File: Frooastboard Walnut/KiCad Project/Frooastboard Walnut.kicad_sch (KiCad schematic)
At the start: 159 parts, among them SW1 SW_Push, U1 ATmega32U4-A, Y1 Crystal_GND24_Small

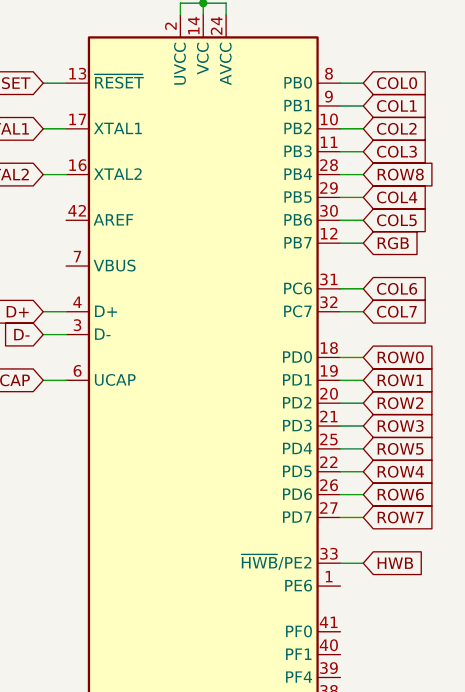
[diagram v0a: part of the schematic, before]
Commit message: backup
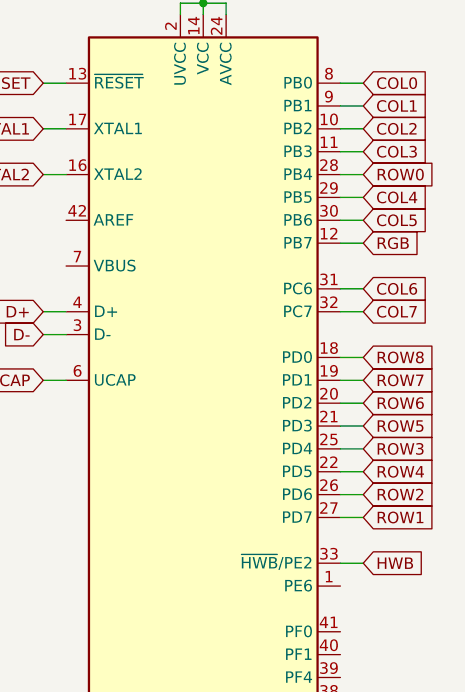
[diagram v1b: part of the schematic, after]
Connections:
- net ROW0: now also U1.28 (PB4); no longer U1.18 (PD0)
- net ROW1: now also U1.27 (PD7); no longer U1.19 (PD1)
- net ROW2: now also U1.26 (PD6); no longer U1.20 (PD2)
- net ROW3: now also U1.25 (PD4); no longer U1.21 (PD3)
- net ROW5: now also U1.21 (PD3); no longer U1.25 (PD4)
- net ROW6: now also U1.20 (PD2); no longer U1.26 (PD6)
- net ROW7: now also U1.19 (PD1); no longer U1.27 (PD7)
- net ROW8: now also U1.18 (PD0); no longer U1.28 (PB4)

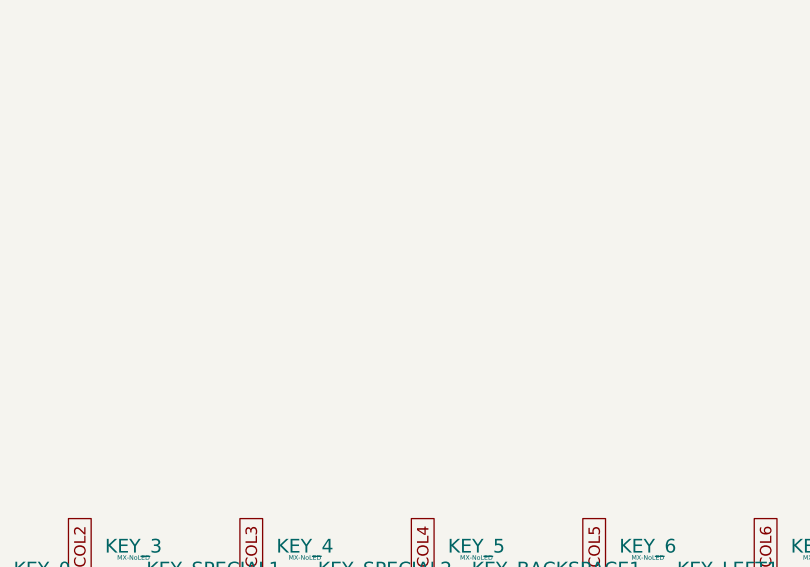
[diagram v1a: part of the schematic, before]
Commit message: Finished Basic Layout
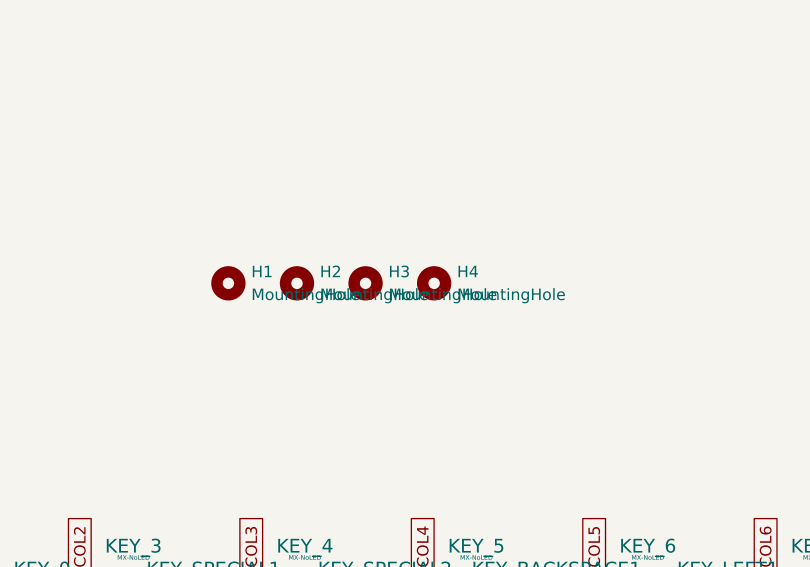
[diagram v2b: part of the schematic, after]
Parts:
- added H1, H2, H3, H4: MountingHole, MountingHole:MountingHole_3.2mm_M3_DIN965, symbol Mechanical:MountingHole
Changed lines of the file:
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@@
     (pin "2")
+  )
+  (symbol (lib_id "Mechanical:MountingHole") (at 116.84 74.93 0) (unit 1)
+    (in_bom yes) (on_board yes) (fields_autoplaced)
+    (property "Reference" "H4" (id 0) (at 119.38 73.6599 0)
+      (effects (font (size 1.27 1.27)) (justify left))
+    )
+    (property "Value" "MountingHole" (id 1) (at 119.38 76.1999 0)
+      (effects (font (size 1.27 1.27)) (justify left))
+    )
+    (property "Footprint" "MountingHole:MountingHole_3.2mm_M3_DIN965" (id 2) (at 116.84 74.93 0)
+      (effects (font (size 1.27 1.27)) hide)
+    )
+    (property "Datasheet" "~" (id 3) (at 116.84 74.93 0)
+      (effects (font (size 1.27 1.27)) hide)
+    )
   )
   (symbol (lib_id "MX_Alps_Hybrid:MX-NoLED") (at 139.7 163.83 0) (unit 1)
@@
     (pin "2")
   )
+  (symbol (lib_id "Mechanical:MountingHole") (at 101.6 74.93 0) (unit 1)
+    (in_bom yes) (on_board yes) (fields_autoplaced)
+    (property "Reference" "H2" (id 0) (at 104.14 73.6599 0)
+      (effects (font (size 1.27 1.27)) (justify left))
+    )
+    (property "Value" "MountingHole" (id 1) (at 104.14 76.1999 0)
+      (effects (font (size 1.27 1.27)) (justify left))
+    )
+    (property "Footprint" "MountingHole:MountingHole_3.2mm_M3_DIN965" (id 2) (at 101.6 74.93 0)
+      (effects (font (size 1.27 1.27)) hide)
+    )
+    (property "Datasheet" "~" (id 3) (at 101.6 74.93 0)
+      (effects (font (size 1.27 1.27)) hide)
+    )
+  )
   (symbol (lib_id "MX_Alps_Hybrid:MX-NoLED") (at 72.39 113.03 0) (unit 1)
     (in_bom yes) (on_board yes) (fields_autoplaced)
@@
     (pin "2")
   )
+  (symbol (lib_id "Mechanical:MountingHole") (at 93.98 74.93 0) (unit 1)
+    (in_bom yes) (on_board yes) (fields_autoplaced)
+    (property "Reference" "H1" (id 0) (at 96.52 73.6599 0)
+      (effects (font (size 1.27 1.27)) (justify left))
+    )
+    (property "Value" "MountingHole" (id 1) (at 96.52 76.1999 0)
+      (effects (font (size 1.27 1.27)) (justify left))
+    )
+    (property "Footprint" "MountingHole:MountingHole_3.2mm_M3_DIN965" (id 2) (at 93.98 74.93 0)
+      (effects (font (size 1.27 1.27)) hide)
+    )
+    (property "Datasheet" "~" (id 3) (at 93.98 74.93 0)
+      (effects (font (size 1.27 1.27)) hide)
+    )
+  )
   (symbol (lib_id "Device:D_Small") (at 71.12 120.65 90) (unit 1)
     (in_bom yes) (on_board yes) (fields_autoplaced)
@@
     (pin "1")
     (pin "2")
+  )
+  (symbol (lib_id "Mechanical:MountingHole") (at 109.22 74.93 0) (unit 1)
+    (in_bom yes) (on_board yes) (fields_autoplaced)
+    (property "Reference" "H3" (id 0) (at 111.76 73.6599 0)
+      (effects (font (size 1.27 1.27)) (justify left))
+    )
+    (property "Value" "MountingHole" (id 1) (at 111.76 76.1999 0)
+      (effects (font (size 1.27 1.27)) (justify left))
+    )
+    (property "Footprint" "MountingHole:MountingHole_3.2mm_M3_DIN965" (id 2) (at 109.22 74.93 0)
+      (effects (font (size 1.27 1.27)) hide)
+    )
+    (property "Datasheet" "~" (id 3) (at 109.22 74.93 0)
+      (effects (font (size 1.27 1.27)) hide)
+    )
   )
   (symbol (lib_id "Device:D_Small") (at 138.43 118.11 90) (unit 1)
@@
       (reference "D72") (unit 1) (value "D_Small") (footprint "Diode_SMD:D_0805_2012Metric")
     )
+    (path "/e7b0a333-0b36-4b50-8f46-39a6d67d5094"
+      (reference "H1") (unit 1) (value "MountingHole") (footprint "MountingHole:MountingHole_3.2mm_M3_DIN965")
+    )
+    (path "/cad75c88-1662-4ffe-80d2-7302cd92fc82"
+      (reference "H2") (unit 1) (value "MountingHole") (footprint "MountingHole:MountingHole_3.2mm_M3_DIN965")
+    )
+    (path "/ed1dc1a0-c3af-4b4a-8e9a-7a16d9c5e1d5"
+      (reference "H3") (unit 1) (value "MountingHole") (footprint "MountingHole:MountingHole_3.2mm_M3_DIN965")
+    )
+    (path "/4f958d36-95b6-4faf-a407-6ffdc897b0c5"
+      (reference "H4") (unit 1) (value "MountingHole") (footprint "MountingHole:MountingHole_3.2mm_M3_DIN965")
+    )
     (path "/c8f17c30-a4f6-46fa-aabd-8086ab44b007"

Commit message: tqfp -> qfn
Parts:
- U1: footprint Package_QFP:TQFP-44_10x10mm_P0.8mm -> Package_DFN_QFN:QFN-44-1EP_7x7mm_P0.5mm_EP5.2x5.2mm
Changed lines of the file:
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@@
       (effects (font (size 1.27 1.27)) (justify left))
     )
-    (property "Footprint" "Package_QFP:TQFP-44_10x10mm_P0.8mm" (id 2) (at 207.01 73.66 0)
+    (property "Footprint" "Package_DFN_QFN:QFN-44-1EP_7x7mm_P0.5mm_EP5.2x5.2mm" (id 2) (at 207.01 73.66 0)
       (effects (font (size 1.27 1.27) italic) hide)
     )
@@
     )
     (path "/20d6f2ba-982f-4f6c-b65d-ffaec9a20f50"
-      (reference "U1") (unit 1) (value "ATmega32U4-A") (footprint "Package_QFP:TQFP-44_10x10mm_P0.8mm")
+      (reference "U1") (unit 1) (value "ATmega32U4-A") (footprint "Package_DFN_QFN:QFN-44-1EP_7x7mm_P0.5mm_EP5.2x5.2mm")
     )
     (path "/aab2d817-6308-4a4a-beb4-4d42d4203987"

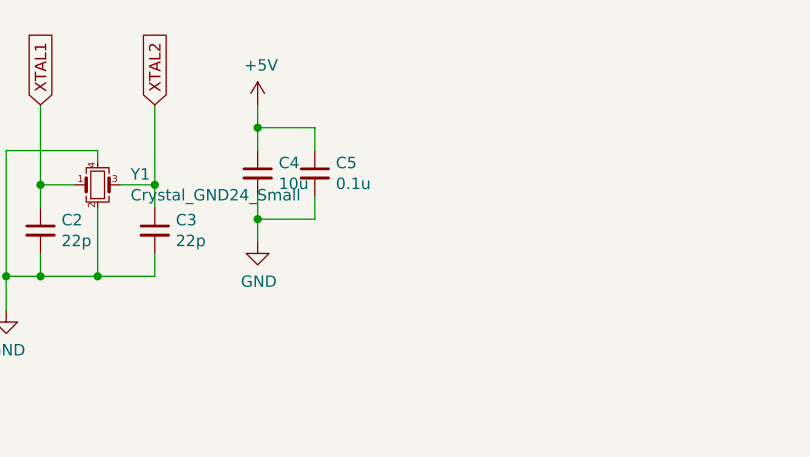
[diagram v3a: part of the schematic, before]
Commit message: update
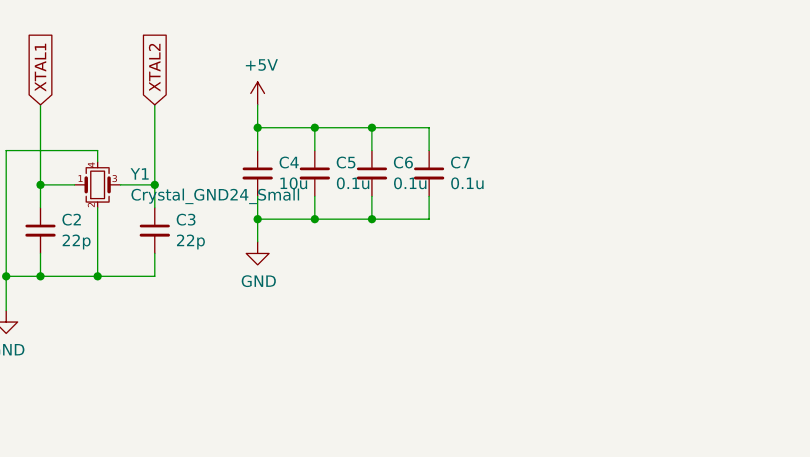
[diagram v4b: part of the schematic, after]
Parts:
- added C6, C7: 0.1u, Capacitor_SMD:C_0805_2012Metric, symbol Device:C_Small
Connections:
- net +5V: now also C6.1, C7.1
- net GND: now also C6.2, C7.2
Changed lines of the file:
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@@
   (junction (at 138.43 193.04) (diameter 0) (color 0 0 0 0)
   )
+  (junction (at 93.98 25.4) (diameter 0) (color 0 0 0 0)
+  )
   (junction (at 81.28 121.92) (diameter 0) (color 0 0 0 0)
   )
@@
   (junction (at 52.07 142.24) (diameter 0) (color 0 0 0 0)
   )
+  (junction (at 100.33 25.4) (diameter 0) (color 0 0 0 0)
+  )
   (junction (at 62.23 121.92) (diameter 0) (color 0 0 0 0)
   )
@@
   (junction (at 39.37 60.96) (diameter 0) (color 0 0 0 0)
   )
+  (junction (at 100.33 35.56) (diameter 0) (color 0 0 0 0)
+  )
   (junction (at 147.32 177.8) (diameter 0) (color 0 0 0 0)
   )
@@
   (junction (at 115.57 127) (diameter 0) (color 0 0 0 0)
   )
+  (junction (at 93.98 35.56) (diameter 0) (color 0 0 0 0)
+  )
   (junction (at 58.42 111.76) (diameter 0) (color 0 0 0 0)
   )
@@
     (stroke (width 0) (type default) (color 0 0 0 0))
   )
+  (wire (pts (xy 106.68 35.56) (xy 106.68 33.02))
+    (stroke (width 0) (type default) (color 0 0 0 0))
+  )
   (wire (pts (xy 48.26 180.34) (xy 58.42 180.34))
     (stroke (width 0) (type default) (color 0 0 0 0))
@@
     (stroke (width 0) (type default) (color 0 0 0 0))
   )
+  (wire (pts (xy 100.33 35.56) (xy 100.33 33.02))
+    (stroke (width 0) (type default) (color 0 0 0 0))
+  )
   (wire (pts (xy 115.57 147.32) (xy 114.3 147.32))
     (stroke (width 0) (type default) (color 0 0 0 0))
@@
     (stroke (width 0) (type default) (color 0 0 0 0))
   )
+  (wire (pts (xy 93.98 35.56) (xy 100.33 35.56))
+    (stroke (width 0) (type default) (color 0 0 0 0))
+  )
   (wire (pts (xy 58.42 165.1) (xy 57.15 165.1))
     (stroke (width 0) (type default) (color 0 0 0 0))
@@
     (stroke (width 0) (type default) (color 0 0 0 0))
   )
+  (wire (pts (xy 106.68 25.4) (xy 106.68 27.94))
+    (stroke (width 0) (type default) (color 0 0 0 0))
+  )
   (wire (pts (xy 96.52 127) (xy 96.52 129.54))
     (stroke (width 0) (type default) (color 0 0 0 0))
@@
     (stroke (width 0) (type default) (color 0 0 0 0))
   )
+  (wire (pts (xy 100.33 25.4) (xy 106.68 25.4))
+    (stroke (width 0) (type default) (color 0 0 0 0))
+  )
   (wire (pts (xy 204.47 120.65) (xy 204.47 121.92))
     (stroke (width 0) (type default) (color 0 0 0 0))
@@
     (stroke (width 0) (type default) (color 0 0 0 0))
   )
+  (wire (pts (xy 100.33 35.56) (xy 106.68 35.56))
+    (stroke (width 0) (type default) (color 0 0 0 0))
+  )
   (wire (pts (xy 77.47 165.1) (xy 76.2 165.1))
     (stroke (width 0) (type default) (color 0 0 0 0))
@@
     (stroke (width 0) (type default) (color 0 0 0 0))
   )
+  (wire (pts (xy 100.33 25.4) (xy 100.33 27.94))
+    (stroke (width 0) (type default) (color 0 0 0 0))
+  )
   (wire (pts (xy 24.13 121.92) (xy 43.18 121.92))
     (stroke (width 0) (type default) (color 0 0 0 0))
@@
     (stroke (width 0) (type default) (color 0 0 0 0))
   )
+  (wire (pts (xy 93.98 25.4) (xy 100.33 25.4))
+    (stroke (width 0) (type default) (color 0 0 0 0))
+  )
   (wire (pts (xy 124.46 180.34) (xy 134.62 180.34))
     (stroke (width 0) (type default) (color 0 0 0 0))
@@
     (pin "2")
   )
+  (symbol (lib_id "Device:C_Small") (at 106.68 30.48 0) (unit 1)
+    (in_bom yes) (on_board yes)
+    (property "Reference" "C7" (id 0) (at 109.0168 29.3116 0)
+      (effects (font (size 1.27 1.27)) (justify left))
+    )
+    (property "Value" "0.1u" (id 1) (at 109.0168 31.623 0)
+      (effects (font (size 1.27 1.27)) (justify left))
+    )
+    (property "Footprint" "Capacitor_SMD:C_0805_2012Metric" (id 2) (at 106.68 30.48 0)
+      (effects (font (size 1.27 1.27)) hide)
+    )
+    (property "Datasheet" "~" (id 3) (at 106.68 30.48 0)
+      (effects (font (size 1.27 1.27)) hide)
+    )
+    (pin "1")
+    (pin "2")
+  )
   (symbol (lib_id "MX_Alps_Hybrid:MX-NoLED") (at 167.64 166.37 0) (unit 1)
     (in_bom yes) (on_board yes) (fields_autoplaced)
@@
     (pin "2")
   )
+  (symbol (lib_id "Device:C_Small") (at 100.33 30.48 0) (unit 1)
+    (in_bom yes) (on_board yes)
+    (property "Reference" "C6" (id 0) (at 102.6668 29.3116 0)
+      (effects (font (size 1.27 1.27)) (justify left))
+    )
+    (property "Value" "0.1u" (id 1) (at 102.6668 31.623 0)
+      (effects (font (size 1.27 1.27)) (justify left))
+    )
+    (property "Footprint" "Capacitor_SMD:C_0805_2012Metric" (id 2) (at 100.33 30.48 0)
+      (effects (font (size 1.27 1.27)) hide)
+    )
+    (property "Datasheet" "~" (id 3) (at 100.33 30.48 0)
+      (effects (font (size 1.27 1.27)) hide)
+    )
+    (pin "1")
+    (pin "2")
+  )
   (symbol (lib_id "power:+5V") (at 49.53 58.42 0) (unit 1)
     (in_bom yes) (on_board yes)
@@
       (reference "C5") (unit 1) (value "0.1u") (footprint "Capacitor_SMD:C_0805_2012Metric")
     )
+    (path "/717ea1f7-11b5-41ec-9faf-146a71003551"
+      (reference "C6") (unit 1) (value "0.1u") (footprint "Capacitor_SMD:C_0805_2012Metric")
+    )
+    (path "/59876205-be10-4744-958f-d88e1e6a4a45"
+      (reference "C7") (unit 1) (value "0.1u") (footprint "Capacitor_SMD:C_0805_2012Metric")
+    )
     (path "/1b31fae3-4c96-4338-9c15-91c3d1cd19fd"
